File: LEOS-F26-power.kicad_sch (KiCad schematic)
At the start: 1 part

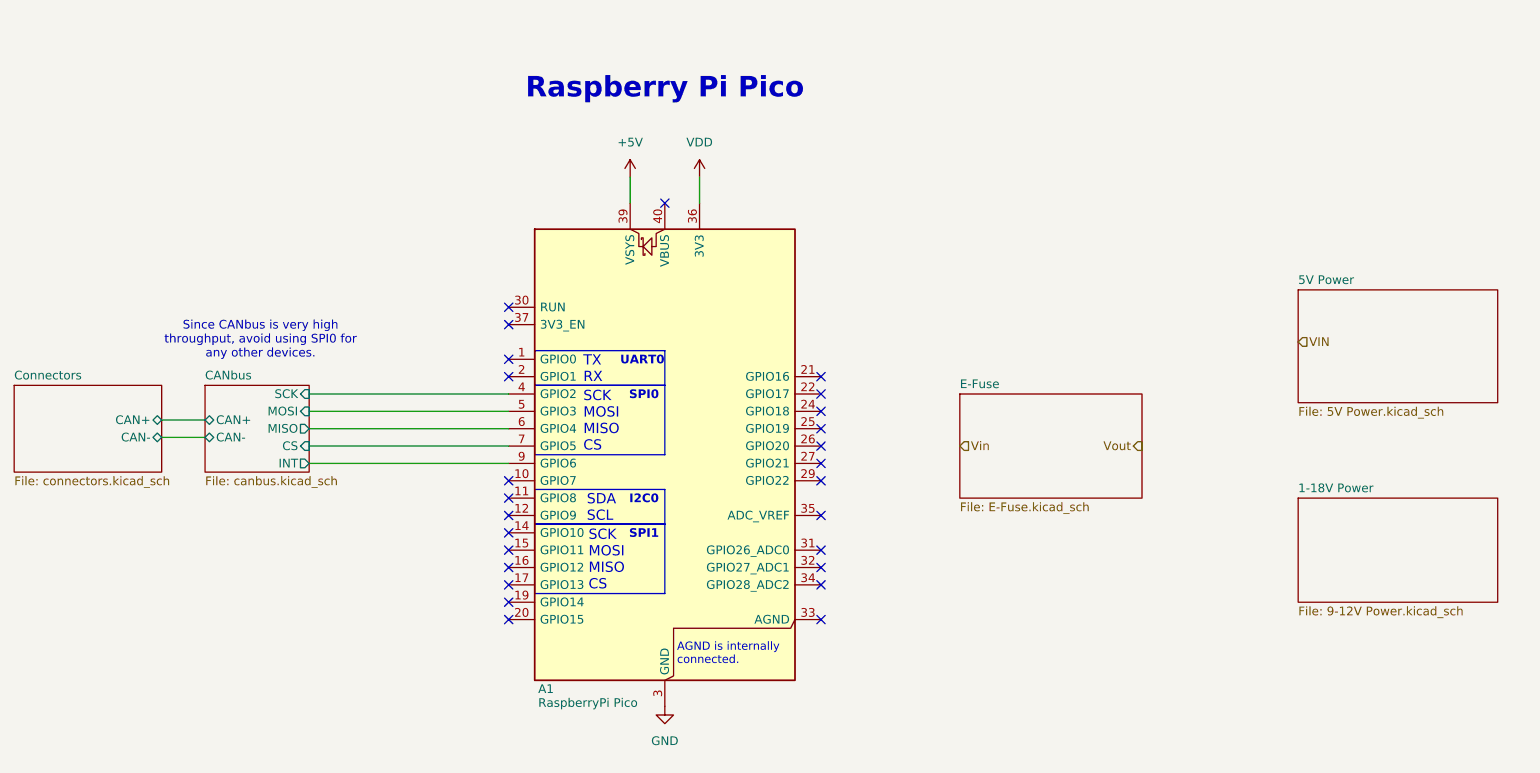
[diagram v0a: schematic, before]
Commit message: updates to potentiometer
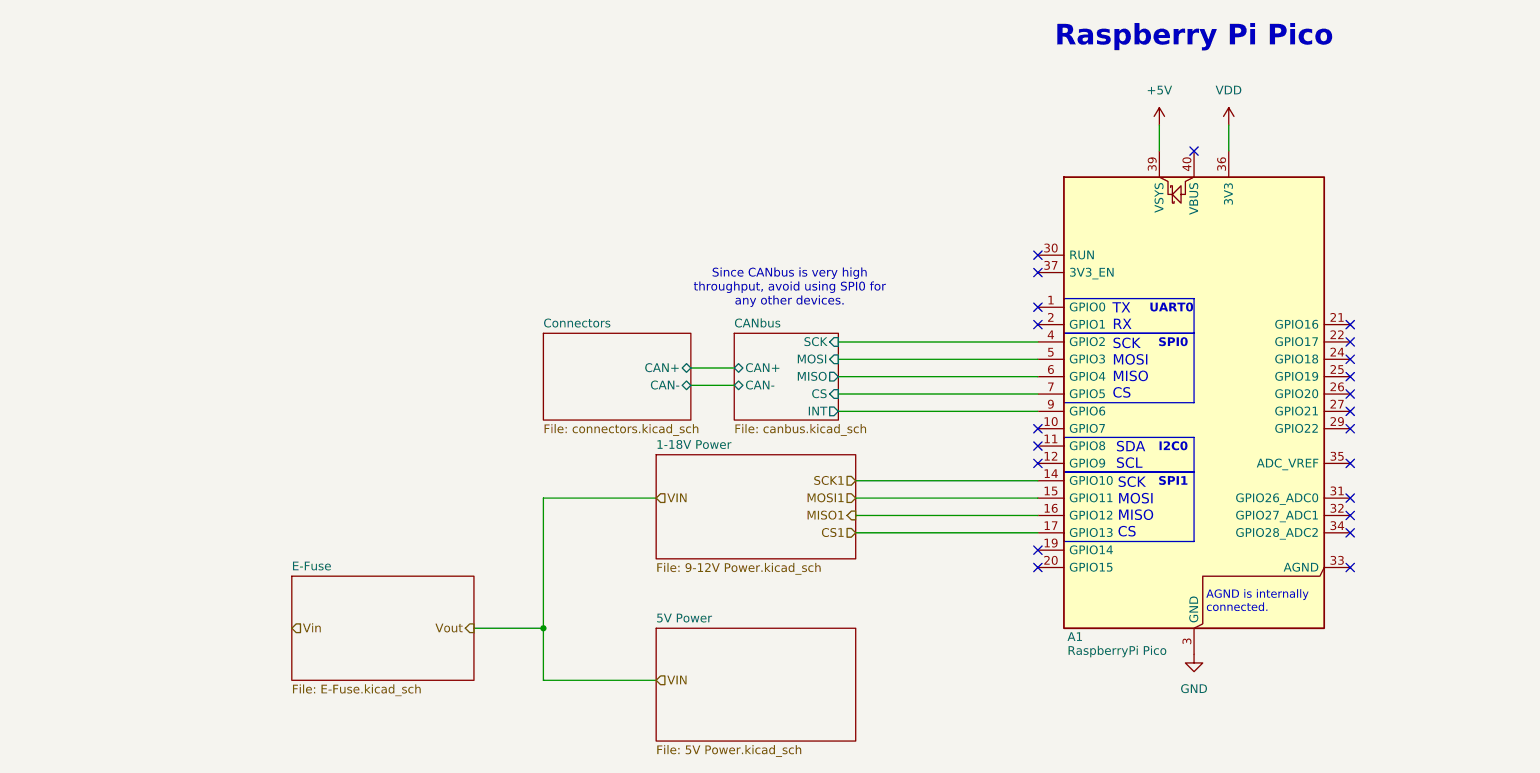
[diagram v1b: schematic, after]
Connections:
- net SCK1: now reaches A1.14 (GPIO10)
- net MOSI1: now reaches A1.15 (GPIO11)
- net MISO1: now reaches A1.16 (GPIO12)
- net CS1: now reaches A1.17 (GPIO13)
- no-connect marks 26 -> 22
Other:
- moved on the sheet: A1
